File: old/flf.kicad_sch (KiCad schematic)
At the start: 70 parts, among them IC1 TB6612FNG, J1 Conn_01x04_Pin, J2 XT30UPB-M, J3 Conn_01x02_Socket, J4 Conn_01x02_Socket, U1 STM32F411CEUx, U10 QRE1113GR, U11 QRE1113GR, U2 TCRT5000L, U3 QRE1113GR, U4 QRE1113GR, U5 QRE1113GR, U6 QRE1113GR, U7 QRE1113GR, U8 QRE1113GR, U9 QRE1113GR, Y1 Crystal

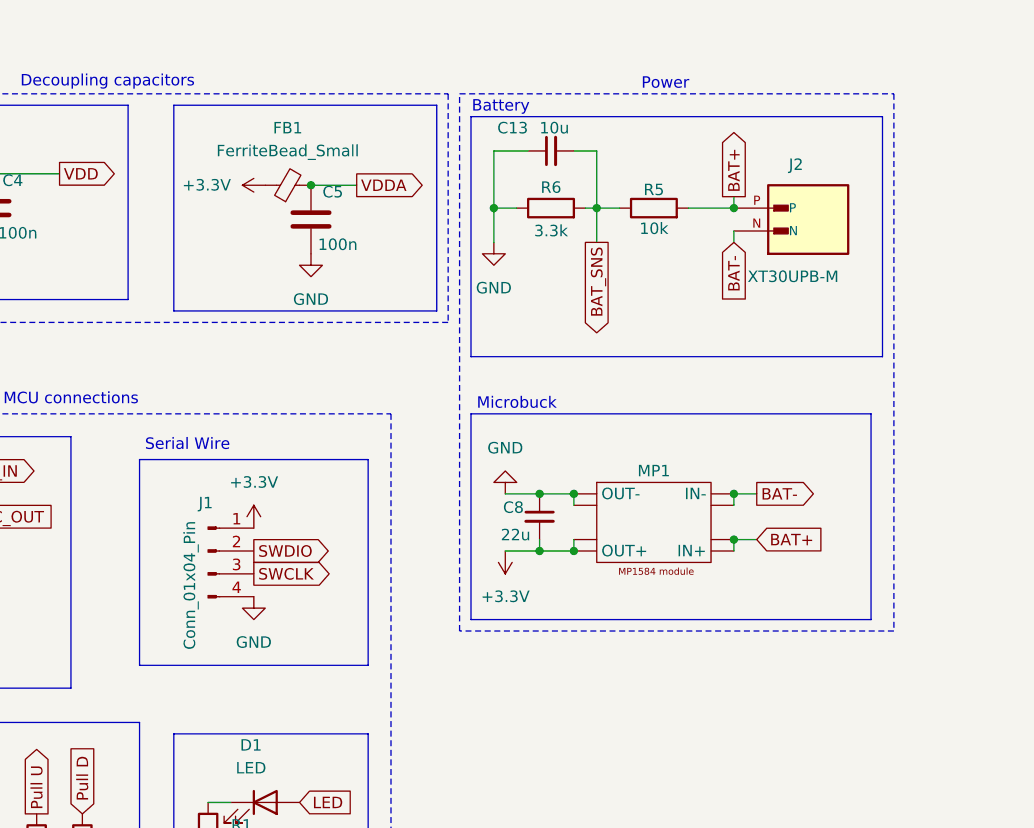
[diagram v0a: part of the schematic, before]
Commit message: new
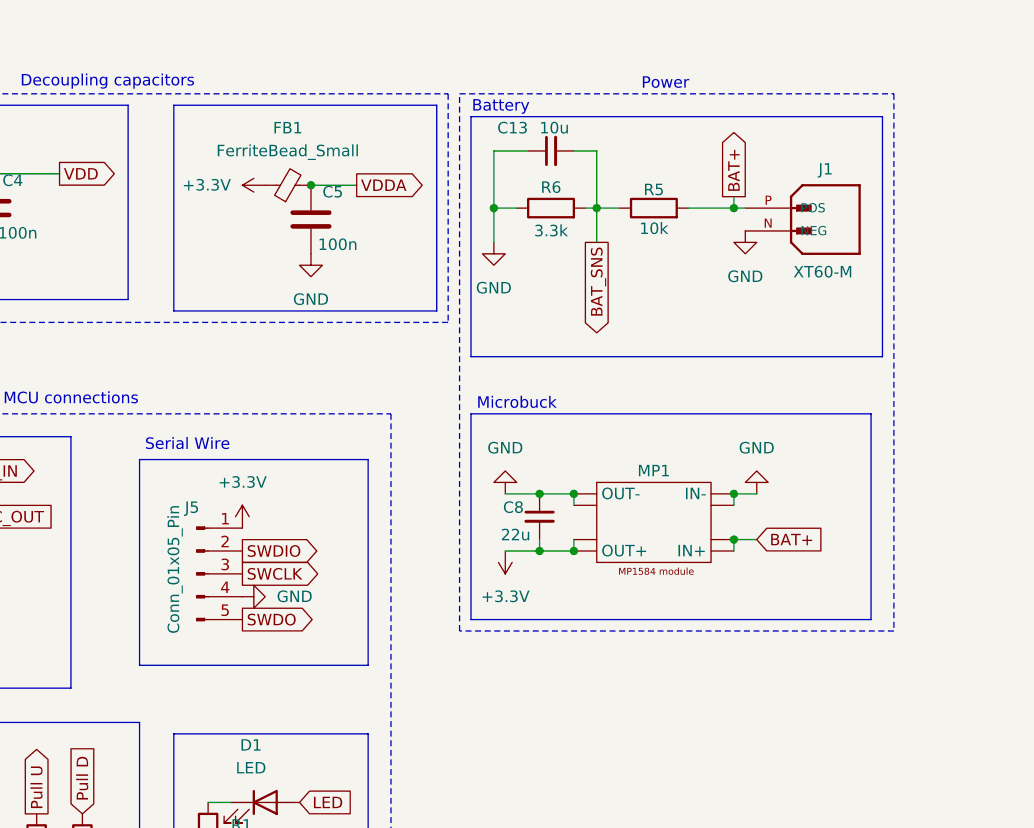
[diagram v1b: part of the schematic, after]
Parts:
- removed J1: Conn_01x04_Pin, symbol Connector:Conn_01x04_Pin
- removed J2: XT30UPB-M, XT30UPB-M:AMASS_XT30UPB-M, symbol customs:XT30UPB-M
- added J1: XT60-M, XT60-M:AMASS_XT60-M, symbol New_Library:XT60-M
- added J5: Conn_01x05_Pin, symbol Connector:Conn_01x05_Pin
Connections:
- net +3.3V: now also J5.1 (Pin_1)
- net BAT+: now also J1.P (POS)
- net BAT-: no longer MP1. (IN+)
- net GND: now also J1.N (NEG), J5.4 (Pin_4)
- net SWCLK: now also J5.3 (Pin_3)
- net SWDIO: now also J5.2 (Pin_2)
- new net SWDO: J5.5 (Pin_5)
